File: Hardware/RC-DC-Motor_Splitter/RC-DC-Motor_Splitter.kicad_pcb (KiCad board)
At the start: 2 copper layers, 38.7 x 17.7 mm, 17 parts, among them J1 Conn_01x01, J10 Conn_01x02, J11 Conn_01x01, J2 Conn_01x02, J3 Conn_01x02, J4 Conn_01x02, J5 Conn_01x02, J6 Conn_01x01, J7 Conn_01x02, J8 Conn_01x02, J9 Conn_01x02, SW1 SW_DIP_x04, U1 ATtiny416-S, U2 LV8548MC_Dual_HBridge_SOIC10, U3 LV8548MC_Dual_HBridge_SOIC10, U4 LV8548MC_Dual_HBridge_SOIC10

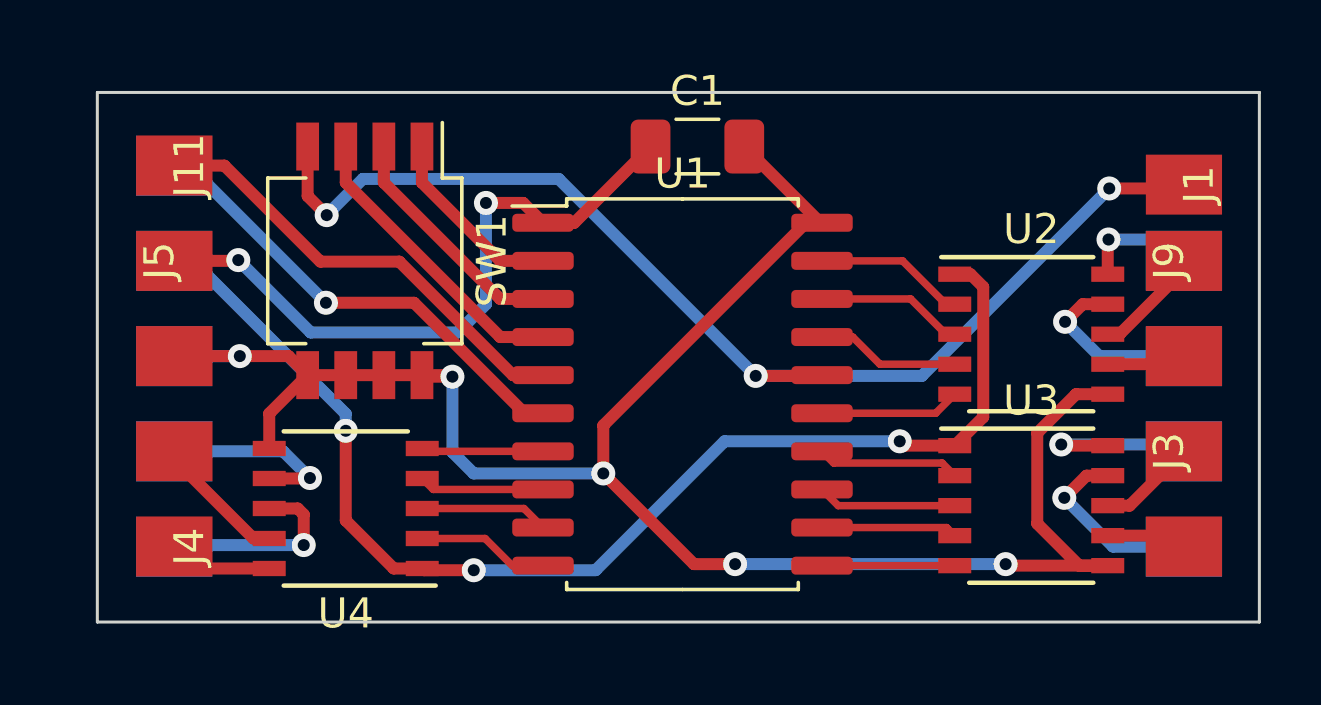
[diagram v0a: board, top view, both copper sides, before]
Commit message: Production Design
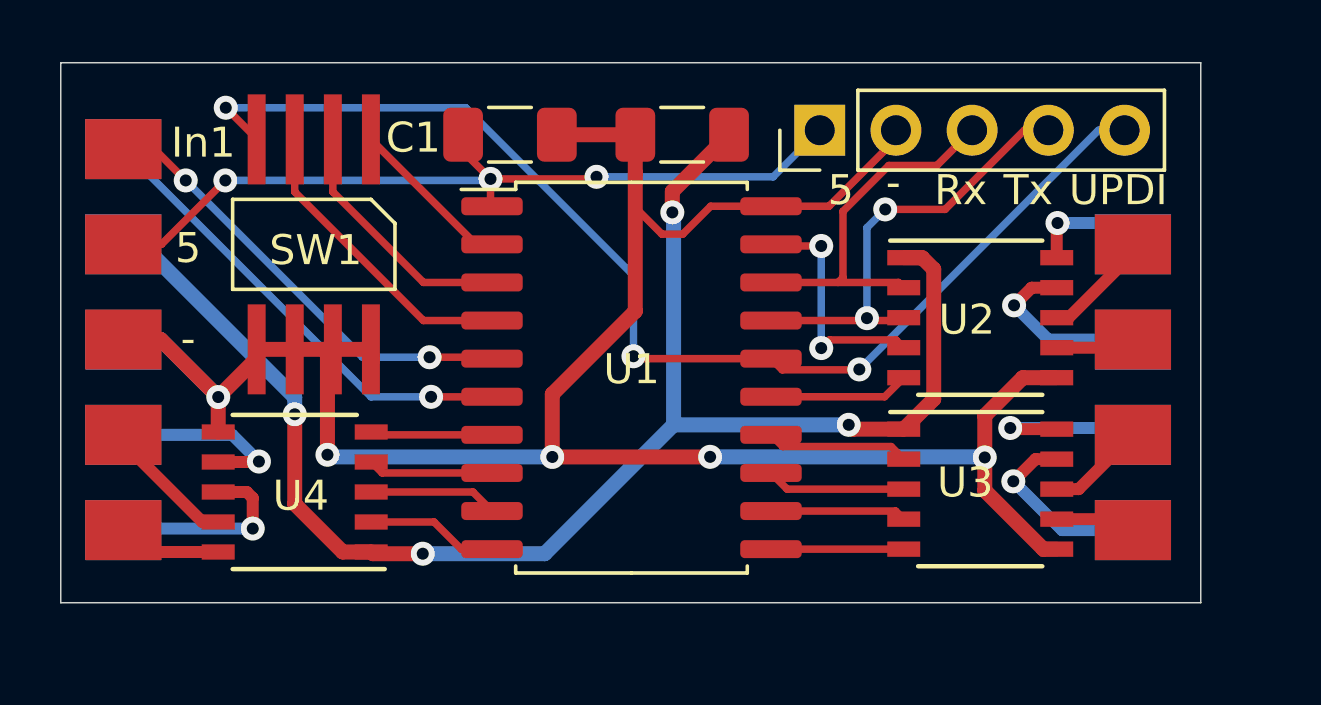
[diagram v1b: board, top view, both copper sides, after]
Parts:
- added C2: 2.2uf, Capacitor_SMD:C_1206_3216Metric_Pad1.33x1.80mm_HandSolder, F.Cu at (111.5, 79.0)
- J1: value Conn_01x01 -> Conn_01x05; footprint RC-DC-Motor_Splitter_footprints:Single_Pad -> Connector_PinHeader_2.54mm:PinHeader_1x05_P2.54mm_Vertical
- SW1: footprint Button_Switch_SMD:SW_DIP_SPSTx04_Slide_Copal_CHS-04B_W7.62mm_P1.27mm -> RC-DC-Motor_Splitter_footprints:SOIC-8-Extended_pads_dip-switch
- moved J1 12.3 mm to (116.1, 78.8)
- moved C1 6.26 mm to (105.8, 79.0)
- moved J2 1.79 mm to (126.6, 89.0)
- moved J3 1.79 mm to (126.6, 89.0)
- moved J7 1.79 mm to (126.6, 82.6)
- moved J9 1.79 mm to (126.6, 82.6)
- moved SW1 1.79 mm to (99.3, 82.6), turned to 180 degrees
- moved U1 1.79 mm to (109.9, 87.1)
- moved U2 1.79 mm to (121.5, 85.1)
- moved U3 1.79 mm to (121.5, 90.8)
- moved U4 1.79 mm to (98.6, 90.9)
- moved J11 1.79 mm to (92.9, 79.5)
- moved J6 1.79 mm to (92.9, 79.5)
- moved J10 1.79 mm to (92.9, 82.6)
- moved J4 1.79 mm to (92.9, 92.2)
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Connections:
- J1 pad 1: UPDI -> +5V
- U1 pad 17: Motor2_In1 -> Motor1_In2
- U1 pad 18: Motor1_In2 -> Motor1_In1
- U1 pad 19: Motor1_In1 -> Motor2_In1
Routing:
- net +12V: track 41.0 -> 51.6 mm, vias 3 -> 4
- net Motor1_In2: track 4.91 -> 15.2 mm, vias 0 -> 2
- net GND: track 65.8 -> 75.8 mm
- net Motor1_In1: track 5.02 -> 12.7 mm
- net +5V: track 22.0 -> 27.6 mm, vias 2 -> 3
- net Motor2_In1: track 4.80 -> 8.13 mm, vias 0 -> 2
- net Input3: track 9.91 -> 11.3 mm
- net Input2: track 8.11 -> 9.51 mm
- net Input1: track 6.32 -> 5.48 mm
- net UPDI: track 39.2 -> 39.9 mm
- net RC_IN1: track 15.8 -> 16.3 mm
- net RC_IN2: vias 0 -> 2
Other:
- board size 38.7 x 17.7 mm -> 38 x 18 mm
- board text added: "+12"
- board text added: "-"
- board text added: "5"
- board text added: "In1"
- board text added: "In2"
- board text added: "M1 --- M2"
- board text added: "M3 --- M4"
- board text added: "M5 --- M6"
- board text added: "R/C-DC Motor Splitter Dom Wilson 2021"
- board text added: "Rx"
- board text added: "Tx"
- board text added: "UPDI"
